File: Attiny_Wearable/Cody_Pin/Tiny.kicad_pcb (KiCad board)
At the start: 2 copper layers, 26.1 x 26.1 mm, 2 parts, among them U2 Codi_Coin

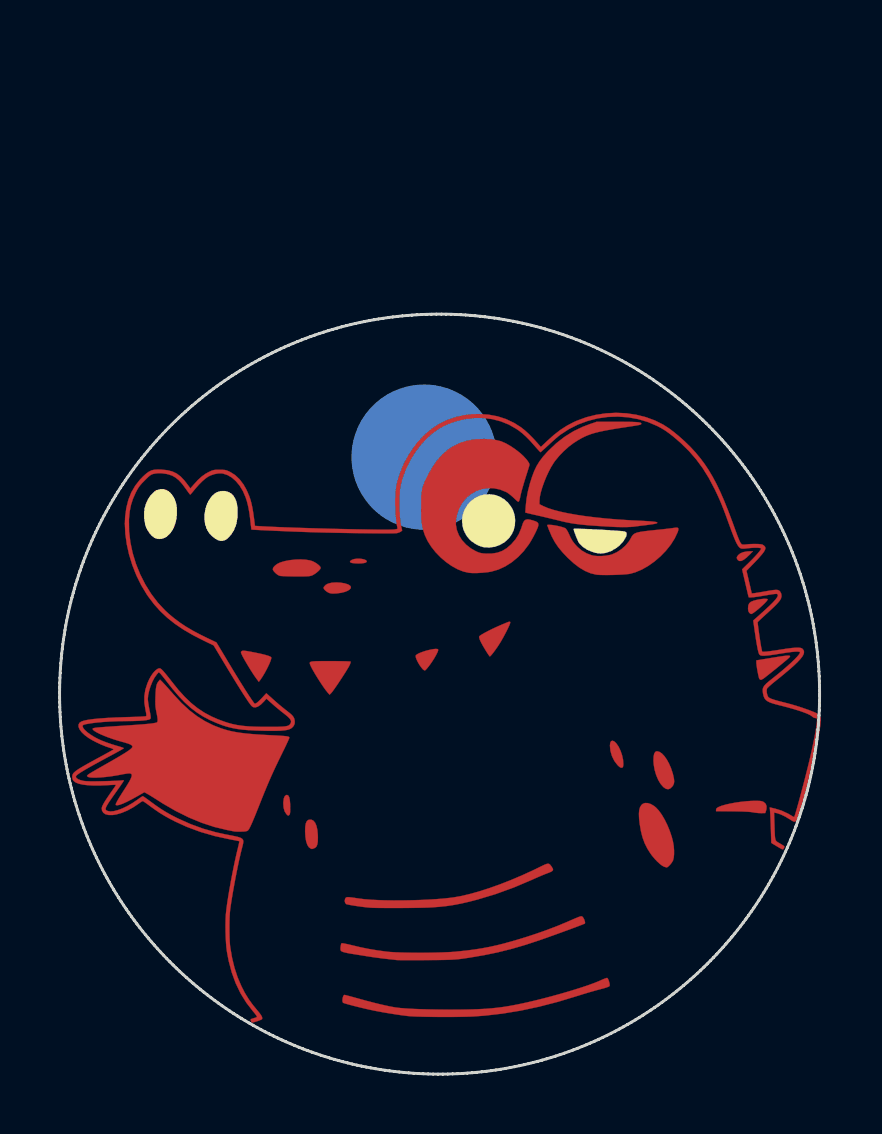
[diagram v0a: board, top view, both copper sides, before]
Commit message: Some changes
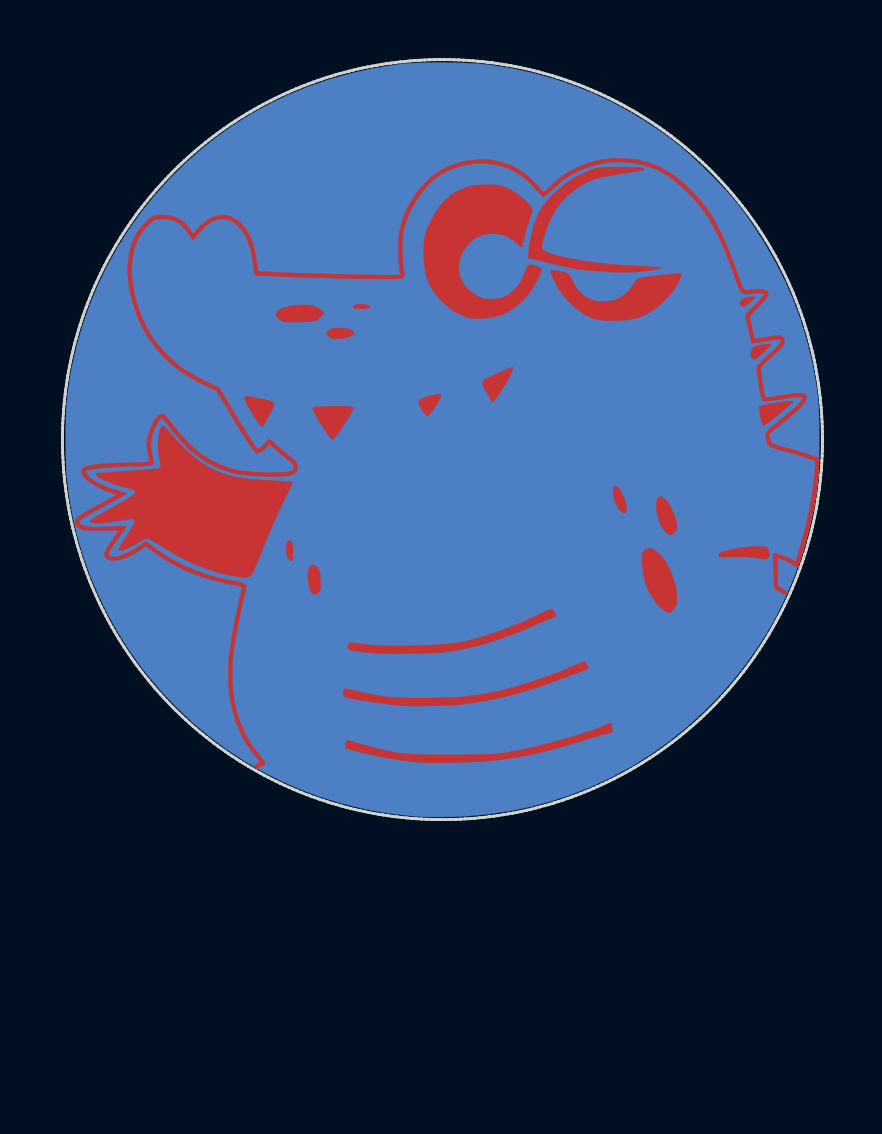
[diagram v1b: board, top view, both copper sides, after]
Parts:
- removed U2: Codi_Coin, Cody_Pin:Cody_Pin
- added Ref**: Val**, Cody_Pin:Cody_Pin_3, F.Cu at (153.0, 74.9)
- moved TP1 5.75 mm to (153.0, 69.8)
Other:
- board text added: "Developed by"
